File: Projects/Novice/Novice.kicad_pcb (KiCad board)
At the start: 2 copper layers, 54.3 x 57 mm, 3 parts

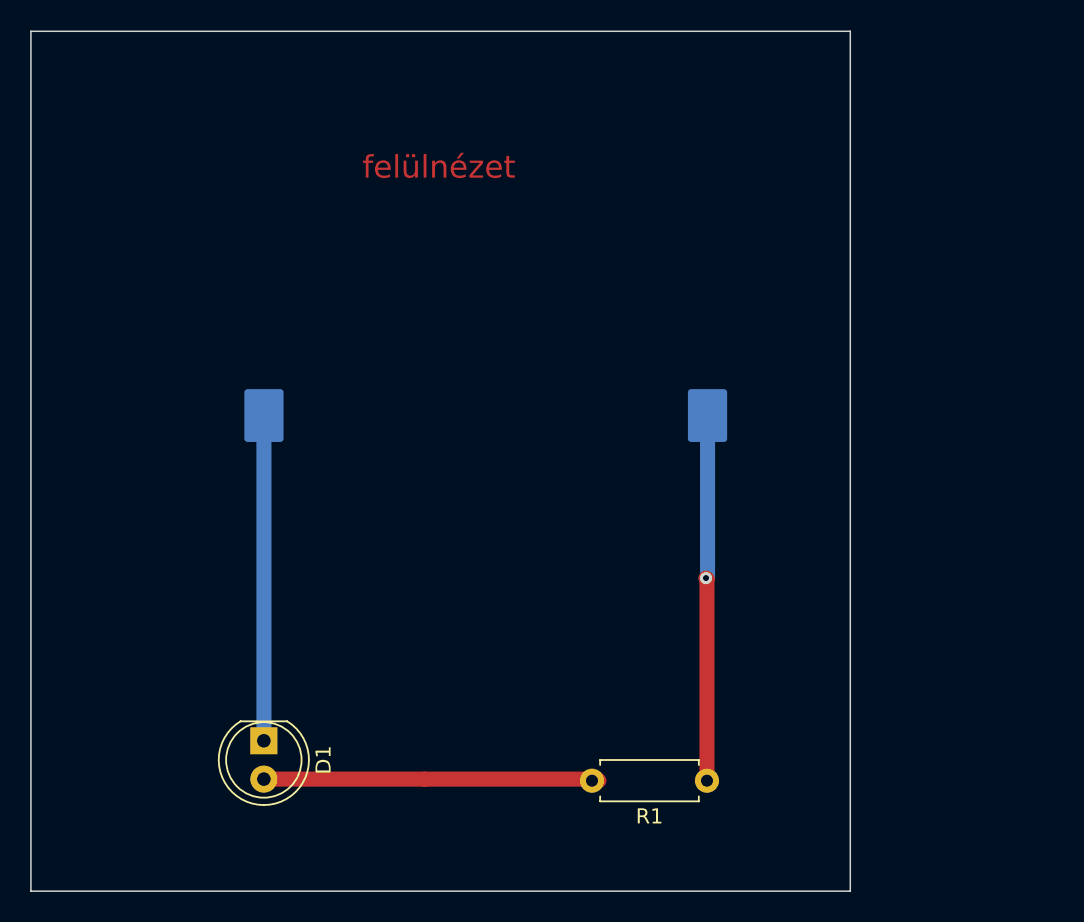
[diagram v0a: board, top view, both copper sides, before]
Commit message: 20240214
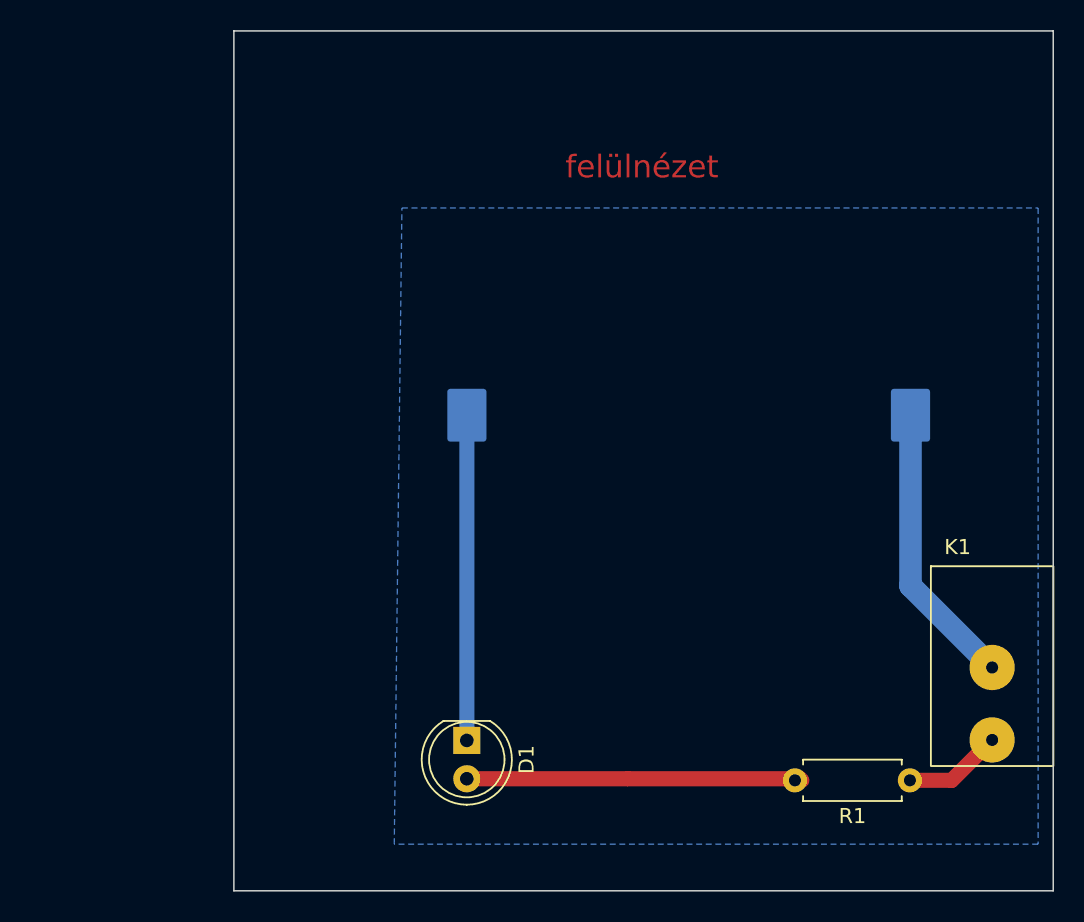
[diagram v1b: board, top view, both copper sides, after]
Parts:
- added K1: M2011S3A1W03, helyi_sajat:kapcsolo, F.Cu at (170.2, 97.8)
- moved D1 13.4 mm to (135.4, 107.4)
- moved BT1 13.4 mm to (150.1, 85.9)
- moved R1 13.4 mm to (164.7, 110.1)
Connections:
- BT1 pad 1: VCC -> Net-(BT1-+)
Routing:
- net Net-(BT1-+): track 0.00 -> 19.0 mm
- net VCC: track 24.3 -> 6.56 mm, vias 1 -> 0
- added copper zone on B.Cu, net GND
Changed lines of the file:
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@@
   (net 2 "GND")
   (net 3 "Net-(D1-A)")
+  (net 4 "Net-(BT1-+)")
   (footprint "LED_THT:LED_D5.0mm" (layer "F.Cu")
-    (at 121.914148 107.447551 -90)
+    (at 135.363749 107.42389 -90)
     (descr "LED, diameter 5.0mm, 2 pins, http://cdn-reichelt.de/documents/datenblatt/A500/LL-504BC2E-009.pdf")
     (tags "LED diameter 5.0mm 2 pins")
@@
     )
   )
+  (footprint "helyi_sajat:kapcsolo" (layer "F.Cu")
+    (at 170.18 97.79)
+    (tags "kapcsolo")
+    (property "Sheetfile" "Novice.kicad_sch")
+    (property "Sheetname" "")
+    (property "ki_keywords" "kapcsoló")
+    (attr through_hole)
+    (fp_text reference "K1" (at -2.29 -3.18 unlocked) (layer "F.SilkS")
+        (effects (font (size 1 1) (thickness 0.15)))
+    )
+    (fp_text value "M2011S3A1W03" (at 0 -0.91 unlocked) (layer "F.Fab")
+        (effects (font (size 1 1) (thickness 0.15)))
+    )
+    (fp_rect (start -4.06 -1.91) (end 4.06 11.33)
+      (stroke (width 0.12) (type default)) (fill none) (layer "F.SilkS"))
+    (fp_rect (start -4.2 -2.05) (end 4.2 11.45)
+      (stroke (width 0.05) (type default)) (fill none) (layer "F.CrtYd"))
+    (fp_rect (start -3.95 -1.8) (end 3.95 11.2)
+      (stroke (width 0.1) (type default)) (fill none) (layer "F.Fab"))
+    (pad "2" thru_hole circle (at 0 4.8) (size 3 3) (drill 0.8) (layers "*.Cu" "*.Mask")
+      (net 4 "Net-(BT1-+)") (pinfunction "A") (pintype "passive"))
+    (pad "3" thru_hole circle (at 0 9.6) (size 3 3) (drill 0.8) (layers "*.Cu" "*.Mask")
+      (net 1 "VCC") (pinfunction "B") (pintype "passive"))
+  )
   (footprint "Resistor_THT:R_Axial_DIN0207_L6.3mm_D2.5mm_P7.62mm_Horizontal" (layer "F.Cu")
-    (at 151.281433 110.091471 180)
+    (at 164.731034 110.06781 180)
     (descr "Resistor, Axial_DIN0207 series, Axial, Horizontal, pin pitch=7.62mm, 0.25W = 1/4W, length*diameter=6.3*2.5mm^2, http://cdn-reichelt.de/documents/datenblatt/B400/1_4W%23YAG.pdf")
     (tags "Resistor Axial_DIN0207 series Axial Horizontal pin pitch 7.62mm 0.25W = 1/4W length 6.3mm diameter 2.5mm")
@@
   )
   (footprint "Battery:BatteryHolder_Renata_SMTU2032-LF_1x2032" (layer "B.Cu")
-    (at 136.62 85.894103 180)
+    (at 150.069601 85.870442 180)
     (descr "https://www.renata.com/fr/downloads/?product=smtu2032-lf&fileid=6a9833a4d49dfb7b550194fe0f")
     (tags "Renata SMT battery holder coin cell 2032")
@@
       (stroke (width 0.1) (type solid)) (fill none) (layer "B.Fab"))
     (pad "1" smd roundrect (at -14.7 0 180) (size 2.6 3.5) (layers "B.Cu" "B.Paste" "B.Mask") (roundrect_rratio 0.07692307692)
-      (net 1 "VCC") (pinfunction "+") (pintype "passive"))
+      (net 4 "Net-(BT1-+)") (pinfunction "+") (pintype "passive"))
     (pad "2" smd roundrect (at 14.7 0 180) (size 2.6 3.5) (layers "B.Cu" "B.Paste" "B.Mask") (roundrect_rratio 0.07692307692)
       (net 2 "GND") (pinfunction "-") (pintype "passive"))
@@
     )
   )
-  (gr_rect (start 106.477939 60.427109) (end 160.779229 117.412957)
+  (gr_rect (start 119.92754 60.403448) (end 174.22883 117.389296)
     (stroke (width 0.1) (type default)) (fill none) (layer "Edge.Cuts"))
-  (gr_text "felülnézet" (at 128.442506 70.311164) (layer "F.Cu")
+  (gr_text "felülnézet" (at 141.892107 70.287503) (layer "F.Cu")
     (effects (font (size 1.5 1.5) (thickness 0.2)) (justify left bottom))
   )
-  (gr_text "Gyakorló" (at 128.23913 66.650402) (layer "Cmts.User")
+  (gr_text "Gyakorló" (at 141.688731 66.626741) (layer "Cmts.User")
     (effects (font (size 3 3) (thickness 0.15)) (justify left bottom))
   )
-  (segment (start 151.218631 96.664428) (end 151.281433 96.72723) (width 1) (layer "F.Cu") (net 1))
-  (segment (start 151.281433 96.72723) (end 151.281433 110.091471) (width 1) (layer "F.Cu") (net 1))
-  (via (at 151.218631 96.664428) (size 0.8) (drill 0.4) (layers "F.Cu" "B.Cu") (net 1))
-  (segment (start 151.270951 85.943152) (end 151.32 85.894103) (width 1) (layer "B.Cu") (net 1))
-  (segment (start 151.32 85.894103) (end 151.32 96.563059) (width 1) (layer "B.Cu") (net 1))
-  (segment (start 151.32 96.563059) (end 151.218631 96.664428) (width 1) (layer "B.Cu") (net 1))
-  (segment (start 121.92 85.894103) (end 121.92 107.441699) (width 1) (layer "B.Cu") (net 2))
-  (segment (start 121.92 107.441699) (end 121.914148 107.447551) (width 1) (layer "B.Cu") (net 2))
-  (segment (start 143.557513 109.987551) (end 143.661433 110.091471) (width 1) (layer "F.Cu") (net 3))
-  (segment (start 121.914148 109.987551) (end 132.569085 109.987551) (width 1) (layer "F.Cu") (net 3))
-  (segment (start 132.569085 109.987551) (end 143.557513 109.987551) (width 1) (layer "F.Cu") (net 3))
-  (segment (start 144.01641 109.987551) (end 144.12033 110.091471) (width 1) (layer "F.Cu") (net 3))
-  (group "" (id 5846ac93-e410-4239-a369-21da4d354d07)
-    (members
-      126075fb-0691-444a-ad74-4607d6e3836c
-      17efd4a9-37a0-4119-8ccd-c1efbfc4b555
-      18b33a02-e435-4f09-bc1e-33d51421ac77
-      3c273958-004b-47ed-a39c-9862018858e4
-      3ebf5236-7322-48d8-9d3a-053279851906
-      42faf91b-6435-4bc8-b9ce-f9cf3eb30b00
-      42fdc401-c3f6-47a4-8cbc-c6e4c326c418
-      5dde1d44-545c-426f-84ca-aed2893f6952
-      6e356059-4712-4420-8d0e-250df23510e1
-      7413950f-e280-4ca1-90be-b909c22a9056
-      83bf766b-c7a0-4c1f-bc35-9a72f873a25f
-      be1bd765-bbd4-4db7-b438-47f1c2913aa1
-      c2bd4c0c-92bf-49f3-b624-0a03214e2bab
-      cb88fda0-103e-4adc-8e7b-7dab164cb3b5
-      d6632148-5390-4dce-8e07-249c8d13ed24
-      e2f6bda9-4e88-4526-b344-315a92a222c4
-      f07a4b5a-2433-4898-a9cf-10c2e548ca9f
-      fa0062e4-2c6f-4621-868a-1a7335284360
-    )
-  )
+  (segment (start 164.731034 110.06781) (end 167.50219 110.06781) (width 1) (layer "F.Cu") (net 1))
+  (segment (start 167.50219 110.06781) (end 170.18 107.39) (width 1) (layer "F.Cu") (net 1))
+  (segment (start 135.369601 85.870442) (end 135.369601 107.418038) (width 1) (layer "B.Cu") (net 2))
+  (segment (start 135.369601 107.418038) (end 135.363749 107.42389) (width 1) (layer "B.Cu") (net 2))
+  (segment (start 157.007114 109.96389) (end 157.111034 110.06781) (width 1) (layer "F.Cu") (net 3))
+  (segment (start 135.363749 109.96389) (end 146.018686 109.96389) (width 1) (layer "F.Cu") (net 3))
+  (segment (start 146.018686 109.96389) (end 157.007114 109.96389) (width 1) (layer "F.Cu") (net 3))
+  (segment (start 157.466011 109.96389) (end 157.569931 110.06781) (width 1) (layer "F.Cu") (net 3))
+  (segment (start 164.720552 85.919491) (end 164.769601 85.870442) (width 1) (layer "B.Cu") (net 4))
+  (segment (start 164.769601 85.870442) (end 164.769601 97.179601) (width 1.5) (layer "B.Cu") (net 4))
+  (segment (start 164.769601 97.179601) (end 170.18 102.59) (width 1.5) (layer "B.Cu") (net 4))
+  (zone (net 2) (net_name "GND") (layer "B.Cu") (hatch edge 0.5)
+    (connect_pads (clearance 1))
+    (min_thickness 0.25) (filled_areas_thickness no)
+    (fill yes (thermal_gap 0.5) (thermal_bridge_width 0.5))
+    (polygon
+      (pts
+        (xy 131.064 72.136)
+        (xy 173.228 72.136)
+        (xy 173.228 114.3)
+        (xy 130.556 114.3)
+      )
+    )
+  )
